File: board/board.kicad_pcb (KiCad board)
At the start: 2 copper layers, 21 x 13 mm, 1 part

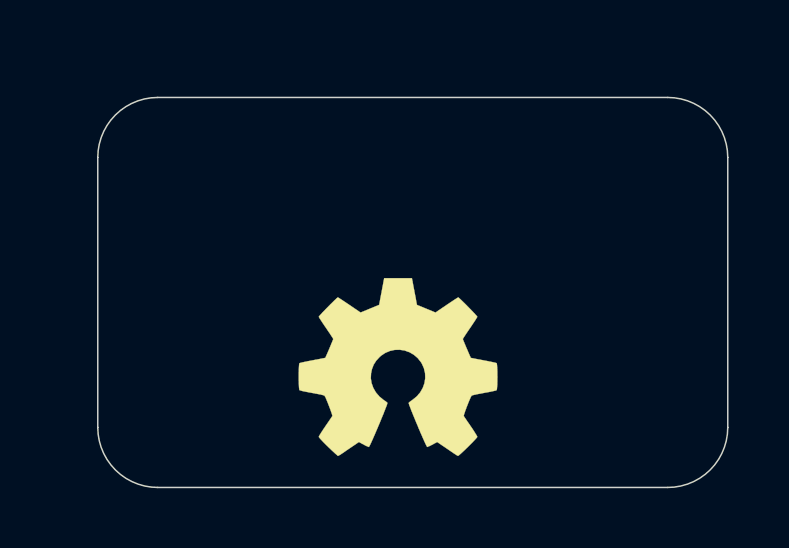
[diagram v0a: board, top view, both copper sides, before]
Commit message: initial commit
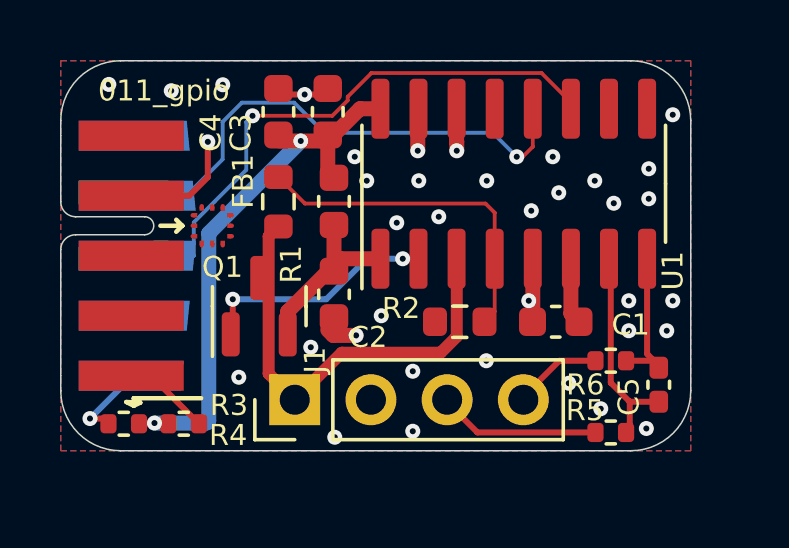
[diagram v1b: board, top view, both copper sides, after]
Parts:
- added C1: 0.1uF, Capacitor_SMD:C_0603_1608Metric, F.Cu at (155.3, 97.5)
- added C2: 0.1uF, Capacitor_SMD:C_0603_1608Metric, F.Cu at (147.9, 96.6)
- added C3: 0.1uF, Capacitor_SMD:C_0603_1608Metric, F.Cu at (147.7, 90.5)
- added C4: 0.1uF, Capacitor_SMD:C_0603_1608Metric, F.Cu at (146.0, 90.5)
- added C5: 0.1uF, Capacitor_SMD:C_0402_1005Metric_Pad0.74x0.62mm_HandSolder, F.Cu at (158.7, 99.6)
- added FB1: >=1k, Inductor_SMD:L_0603_1608Metric, F.Cu at (147.9, 93.5)
- added J1: Conn_01x04_Male, Connector_PinHeader_2.54mm:PinHeader_1x04_P2.54mm_Vertical, F.Cu at (146.6, 100.1)
- added J2: 002_SPI, on_edge:debug_edge_2x05_device, F.Cu at (138.8, 95.3)
- added Q1: BC807, Package_TO_SOT_SMD:SOT-23, F.Cu at (145.4, 97.0)
- added R1: 10k, Resistor_SMD:R_0603_1608Metric, F.Cu at (146.0, 93.5)
- added R2: 10k, Resistor_SMD:R_0603_1608Metric, F.Cu at (152.1, 97.5)
- added R3: 0/DNP, Resistor_SMD:R_0402_1005Metric, F.Cu at (140.9, 100.9)
- added R4: 0/DNP, Resistor_SMD:R_0402_1005Metric, F.Cu at (142.9, 100.9)
- added R5: 100, Resistor_SMD:R_0402_1005Metric, F.Cu at (157.1, 101.2)
- added R6: 100, Resistor_SMD:R_0402_1005Metric, F.Cu at (157.1, 98.8)
- added U1: hx711, hx711_fp:SOP-16_3.9x9.9mm_P1.27mm, F.Cu at (153.9, 92.9)
- LOGO1: moved to B.Cu
- moved LOGO1 4.27 mm to (150.1, 94.7), turned to 180 degrees
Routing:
- net /hx711_hall/PD_SCK: track 0.00 -> 19.7 mm, vias 0 -> 1
- net /hx711_hall/DVDD: track 0.00 -> 18.5 mm, vias 0 -> 2
- net /hx711_hall/DOUT: track 0.00 -> 17.8 mm, vias 0 -> 1
- net /hx711_hall/AVDD: track 0.00 -> 15.1 mm
- net GND: track 0.00 -> 11.5 mm, vias 0 -> 37
- net /hx711_hall/VFB: track 0.00 -> 11.5 mm
- net /hx711_hall/BASE: track 0.00 -> 7.95 mm, vias 0 -> 2
- net Net-(C5-Pad1): track 0.00 -> 7.02 mm
- net /hx711_hall/VSUP: track 0.00 -> 6.12 mm
- net /hx711_hall/INNA: track 0.00 -> 5.23 mm
- net Net-(C5-Pad2): track 0.00 -> 5.20 mm
- net /hx711_hall/VIN: track 0.00 -> 2.92 mm
- net /hx711_hall/INPA: track 0.00 -> 2.77 mm
- net /hx711_hall/VIN_5: track 0.00 -> 2.66 mm, vias 0 -> 1
- net /hx711_hall/VBG: track 0.00 -> 2.21 mm
- added copper zone on B.Cu, net GND
- added copper zone on F.Cu, net GND
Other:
- outline, holes or cut-outs redrawn
- board text added: "011_gpio"
- board text added: "b131_hx711_v1.0"
